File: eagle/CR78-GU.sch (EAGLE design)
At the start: 36 parts, among them Q518 2N3904, Q519 2N3904, Q520 2N3904, Q521 2N3904, Q7 2N3904

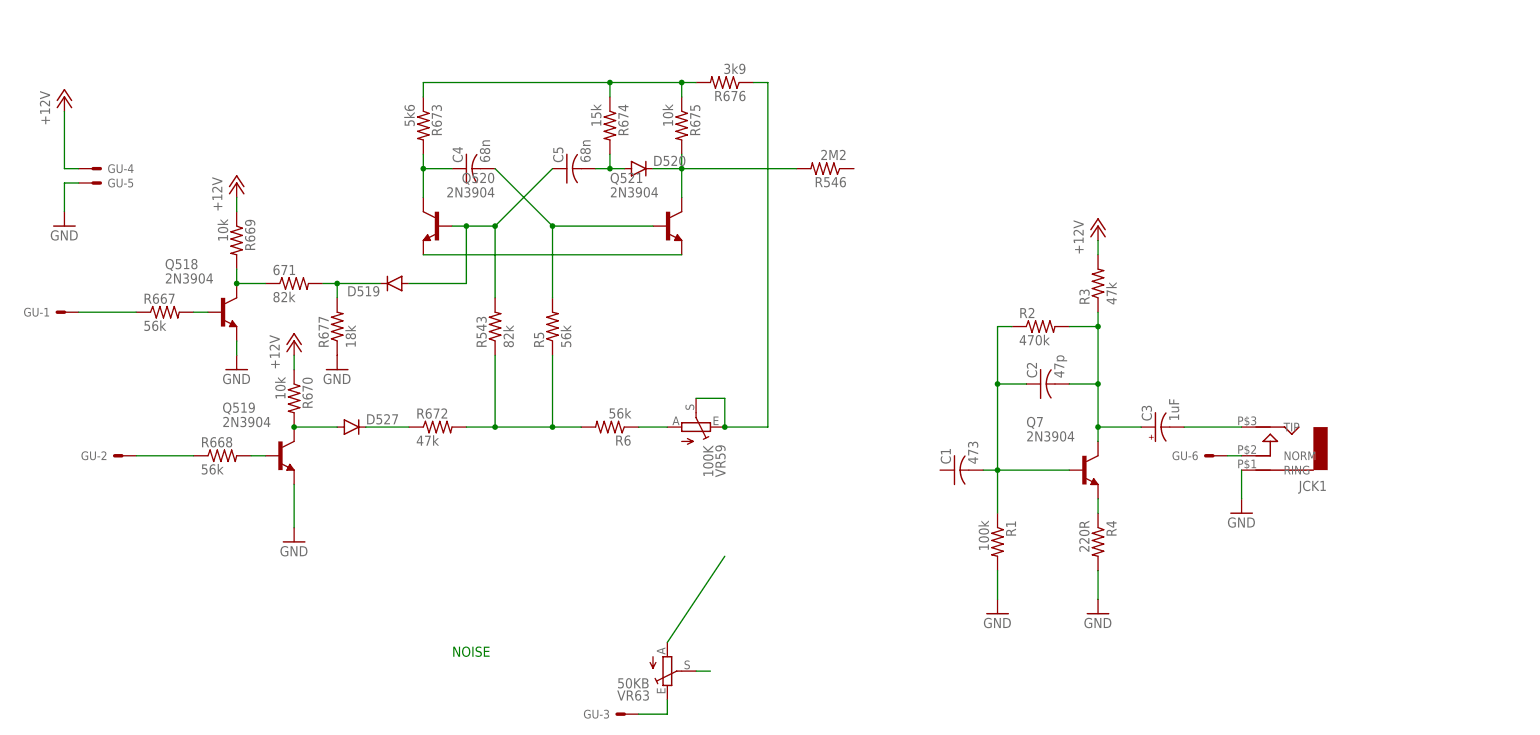
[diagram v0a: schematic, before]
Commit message: schemo in
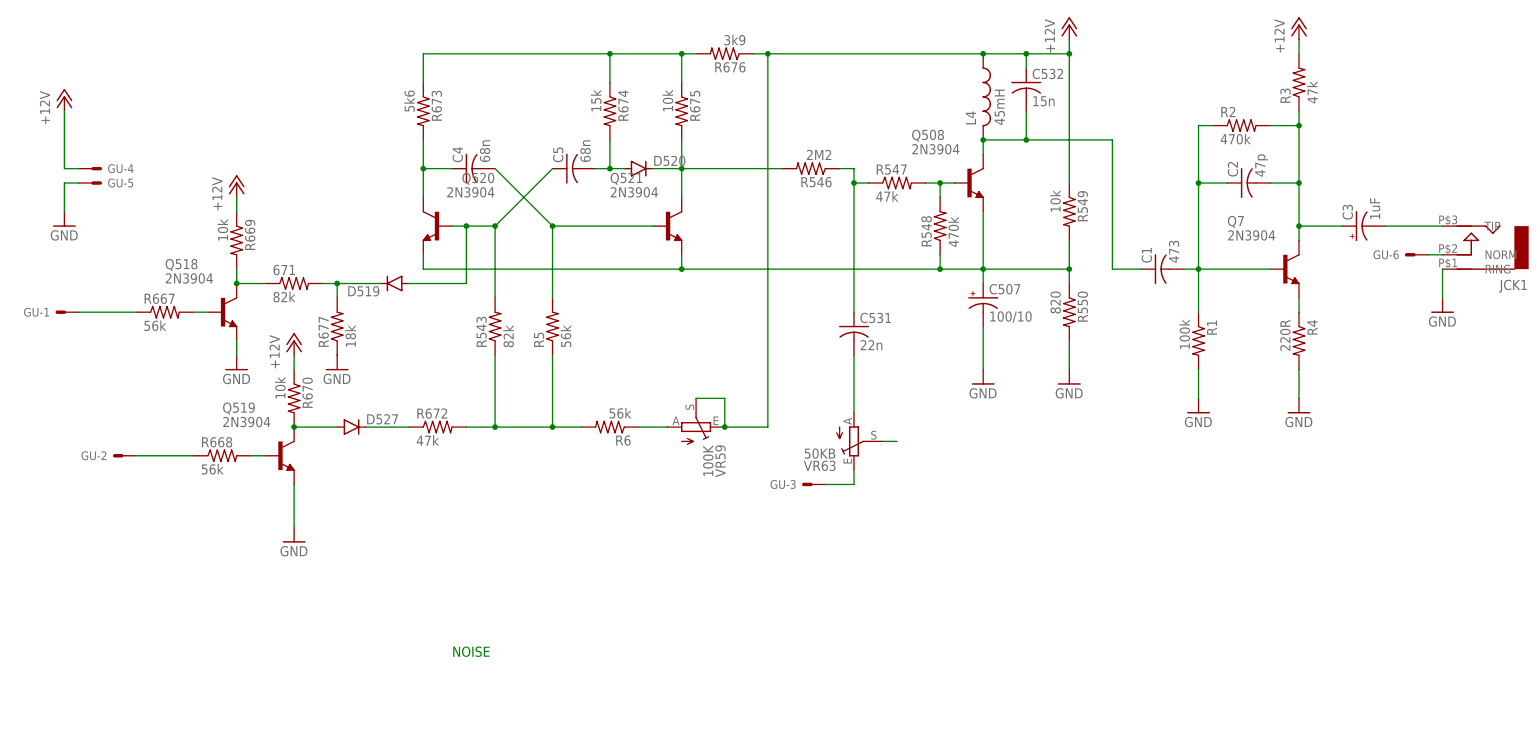
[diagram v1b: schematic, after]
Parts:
- added C507: 100/10, rcl:CPOL-USB45181A
- added C531: 22n, rcl:C-US050-025X075
- added C532: 15n, rcl:C-US050-025X075
- added L4: 45mH, rcl:L-US0204/7
- added Q508: 2N3904, 808_lt:2N3904
- added R547: 47k, rcl:R-US_0207/7
- added R548: 470k, rcl:R-US_0207/7
- added R549: 10k, rcl:R-US_0207/7
- added R550: 820, rcl:R-US_0207/7
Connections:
- new net N$13: Q508.B, R547.2, R548.2
- new net N$27: C1.1, C532.2, L4.2, Q508.C
- net +12V: now also C532.1, L4.1, R549.1, R676.1, VR59.E, VR59.S
- net GND: now also C507.-, R550.2
- net N$12: now also C531.1, R546.1, R547.1; no longer R676.1, VR59.E, VR59.S
- net N$26: now also C531.2
- net N$4: now also C507.+, Q508.E, R548.1, R549.2, R550.1
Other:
- moved on the sheet: C1, C2, C3, GU-3, GU-6, JCK1, Q7, R1, R2, R3, R4, R546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
